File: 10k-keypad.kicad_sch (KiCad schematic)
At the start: 42 parts, among them J1 AVR-ISP-6, K1 SW_Push, K10 SW_Push, K2 SW_Push, K3 SW_Push, K4 SW_Push, K5 SW_Push, K6 SW_Push, K7 SW_Push, K8 SW_Push, K9 SW_Push, SW1 SW_Push, U1 ATmega16U2-A, Y1 Crystal_GND24_Small

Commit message: footprints
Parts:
- C1, C2, C3, C4, C5, C6, C7, C8: footprint (none) -> Capacitor_SMD:C_0805_2012Metric_Pad1.18x1.45mm_HandSolder
- D10, D11, D2, D3, D4, D5, D6, D7, D8, D9: footprint (none) -> Diode_SMD:D_SOD-123
- F1: footprint (none) -> Fuse:Fuse_1206_3216Metric_Pad1.42x1.75mm_HandSolder
- FB1: footprint (none) -> Inductor_SMD:L_0805_2012Metric_Pad1.15x1.40mm_HandSolder
- J1: footprint (none) -> random-keyboard-parts:Reset_Pretty-Mask
- K1, K10, K2, K3, K4, K5, K6, K7, K8, K9: footprint (none) -> marbastlib-mx:SW_MX_HS_CPG151101S11_1u
- R1, R2, R3, R4, R5, R6: footprint (none) -> Resistor_SMD:R_0805_2012Metric_Pad1.20x1.40mm_HandSolder
- SW1: footprint (none) -> Button_Switch_SMD:SW_SPST_SKQG_WithStem
- USB1: footprint (none) -> Type-C:HRO-TYPE-C-31-M-12-HandSoldering
- Y1: footprint (none) -> Crystal:Crystal_SMD_3225-4Pin_3.2x2.5mm_HandSoldering

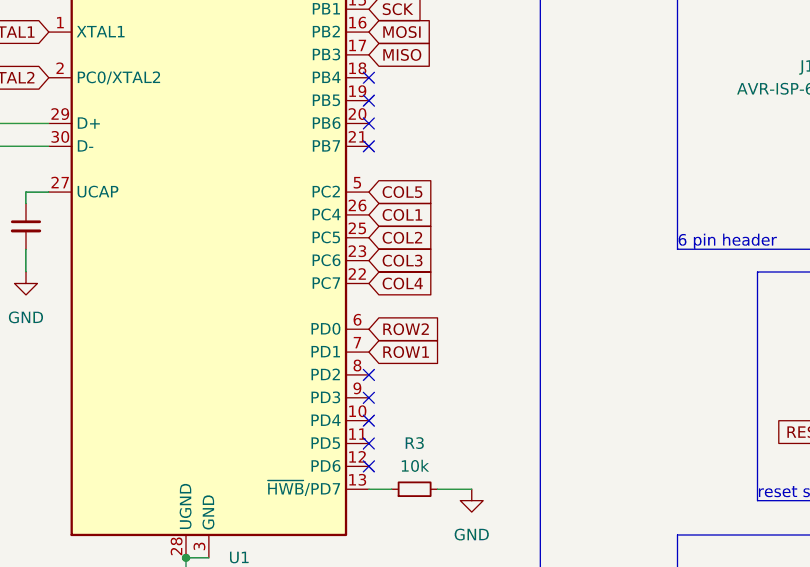
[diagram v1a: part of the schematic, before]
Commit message: crystal clock
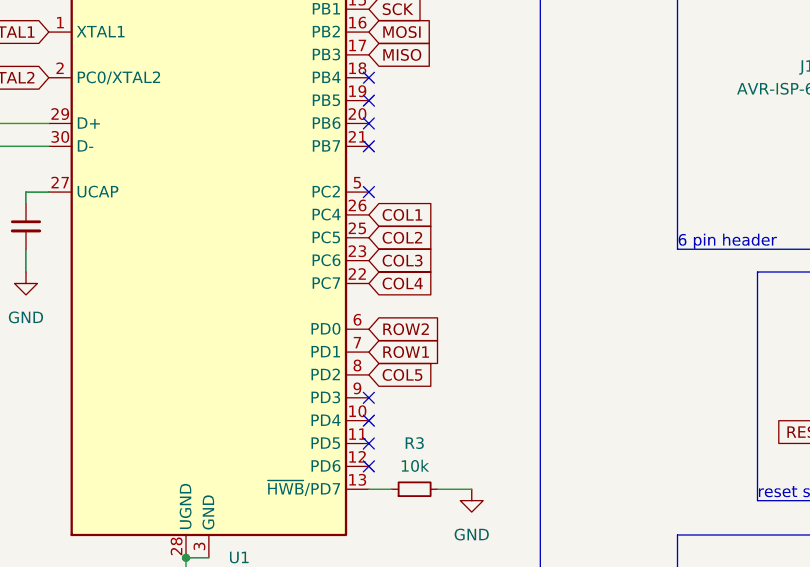
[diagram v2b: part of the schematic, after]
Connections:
- net COL5: now also U1.8 (PD2); no longer U1.5 (PC2)
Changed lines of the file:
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@@
   (no_connect (at 199.39 113.03))
   (no_connect (at 199.39 82.55))
-  (no_connect (at 199.39 110.49))
   (no_connect (at 199.39 85.09))
+  (no_connect (at 199.39 90.17))
   (wire (pts (xy 179.07 59.69) (xy 181.61 59.69))
     (stroke (width 0) (type default))
@@
     )
   )
-  (global_label "COL5" (shape input) (at 199.39 90.17 0) (fields_autoplaced)
-    (effects (font (size 1.27 1.27)) (justify left))
-    (property "Intersheetrefs" "${INTERSHEET_REFS}" (at 207.2133 90.17 0)
-      (effects (font (size 1.27 1.27)) (justify left) hide)
-    )
+  (global_label "COL5" (shape input) (at 199.39 110.49 0) (fields_autoplaced)
+    (effects (font (size 1.27 1.27)) (justify left))
+    (property "Intersheetrefs" "${INTERSHEET_REFS}" (at 207.2133 110.49 0)
+      (effects (font (size 1.27 1.27)) (justify left) hide)
+    )
